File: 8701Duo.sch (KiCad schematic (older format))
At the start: 12 parts, among them J1 Clock, U1 ICS525-01R, U2 MOS8701, U3 74LVC1G06, X1 LFSPXO021772Bulk, X2 LFSPXO020648Bulk

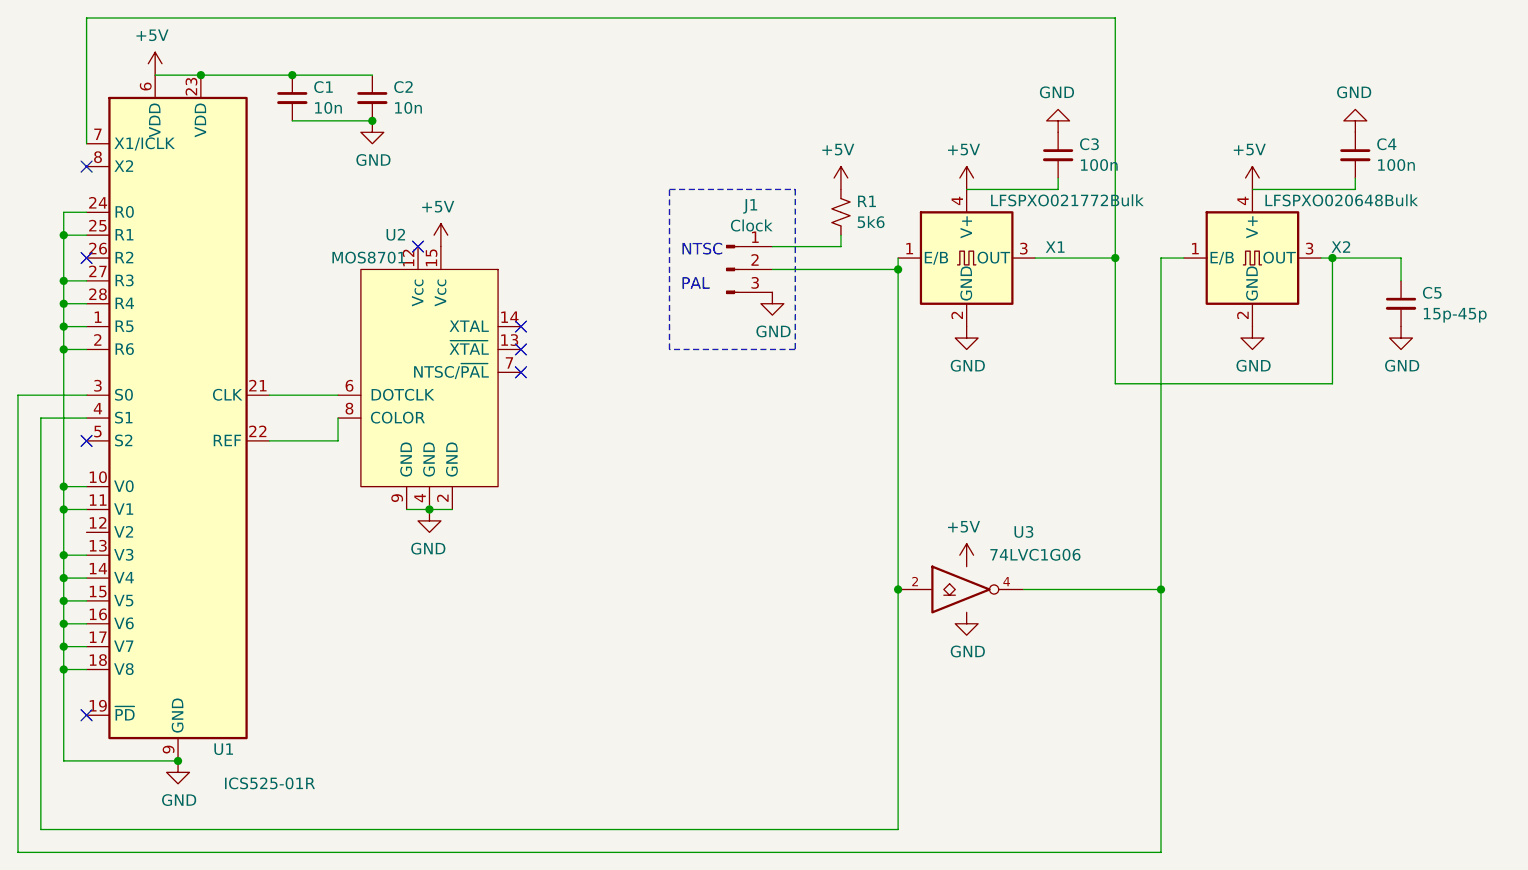
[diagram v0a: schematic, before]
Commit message: Add files via upload
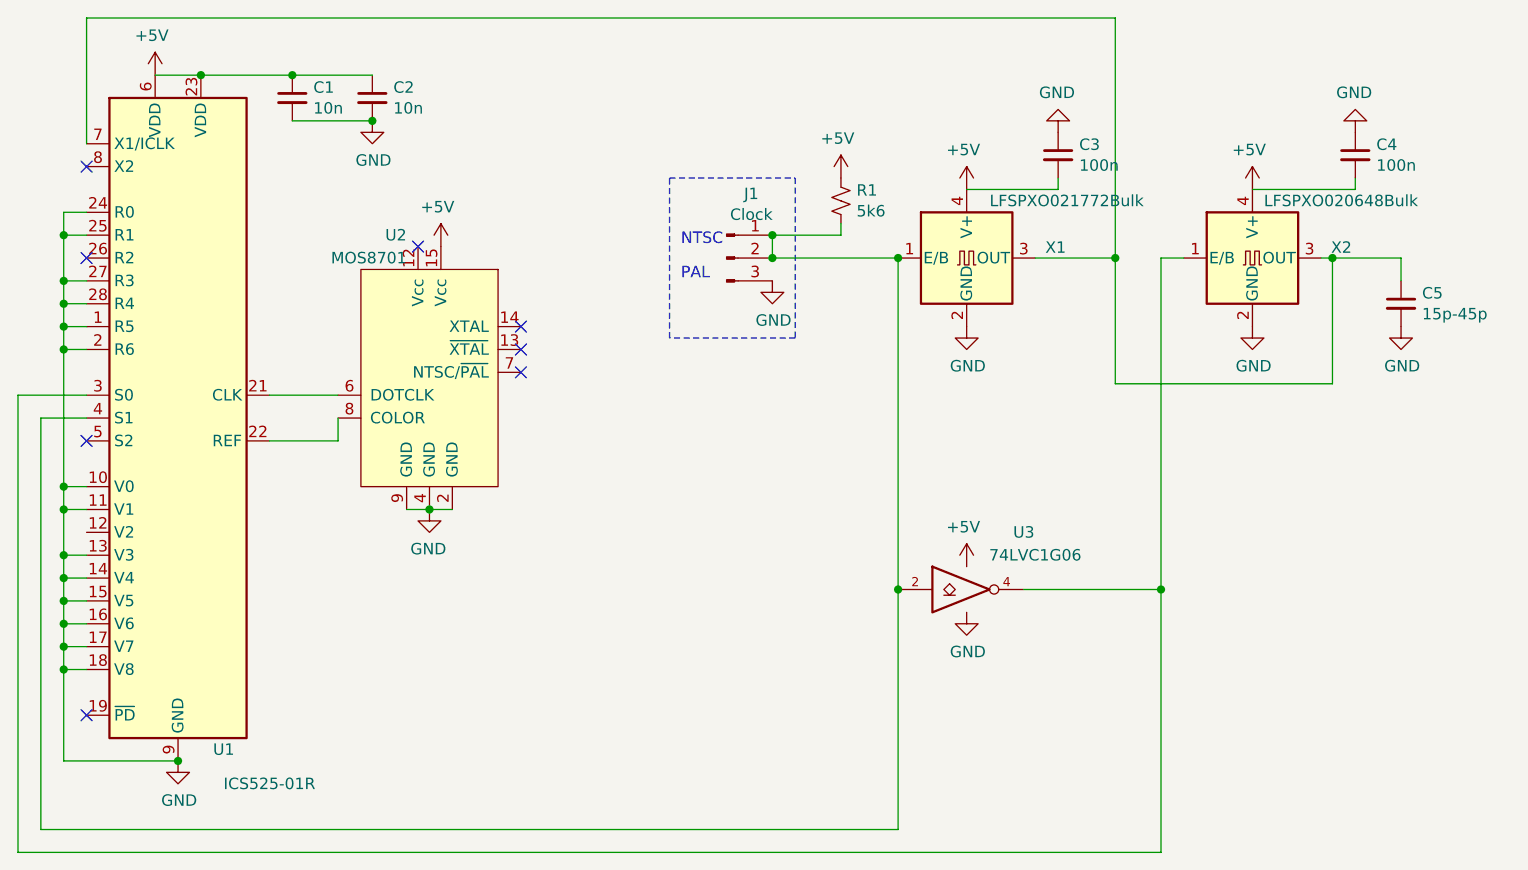
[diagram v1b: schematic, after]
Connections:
- net at J1.2 (Pin_2), U1.4 (S1), U3.2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: now also J1.1 (Pin_1), R1.2
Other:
- moved on the sheet: J1, R1
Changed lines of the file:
@@
 $EndComp
-Wire Wire Line
-	7650 2050 7650 2100
 Wire Wire Line
 	8800 2050 8900 2050
@@
 L Connector:Conn_01x03_Male J1
 U 1 1 5EF16EAC
-P 6900 2100
-F 0 "J1" H 7008 2381 50  0000 C CNN
-F 1 "Clock" H 7008 2290 50  0000 C CNN
-F 2 "Connector_PinHeader_2.54mm:PinHeader_1x03_P2.54mm_Vertical" H 6900 2100 50  0001 C CNN
-F 3 "~" H 6900 2100 50  0001 C CNN
-	1    6900 2100
+P 6900 2050
+F 0 "J1" H 7008 2331 50  0000 C CNN
+F 1 "Clock" H 7008 2240 50  0000 C CNN
+F 2 "Connector_PinHeader_2.54mm:PinHeader_1x03_P2.54mm_Vertical" H 6900 2050 50  0001 C CNN
+F 3 "~" H 6900 2050 50  0001 C CNN
+	1    6900 2050
 	1    0    0    -1
 $EndComp
@@
 L Device:R_Small_US R1
 U 1 1 5EF17D87
-P 7400 1850
-F 0 "R1" H 7468 1896 50  0000 L CNN
-F 1 "5k6" H 7468 1805 50  0000 L CNN
-F 2 "Resistor_SMD:R_0805_2012Metric_Pad1.15x1.40mm_HandSolder" H 7400 1850 50  0001 C CNN
-F 3 "~" H 7400 1850 50  0001 C CNN
-	1    7400 1850
-	1    0    0    -1
-$EndComp
-Wire Wire Line
-	7100 2000 7400 2000
-Wire Wire Line
-	7400 2000 7400 1950
+P 7400 1800
+F 0 "R1" H 7468 1846 50  0000 L CNN
+F 1 "5k6" H 7468 1755 50  0000 L CNN
+F 2 "Resistor_SMD:R_0805_2012Metric_Pad1.15x1.40mm_HandSolder" H 7400 1800 50  0001 C CNN
+F 3 "~" H 7400 1800 50  0001 C CNN
+	1    7400 1800
+	1    0    0    -1
+$EndComp
+Wire Wire Line
+	7100 1950 7400 1950
+Wire Wire Line
+	7400 1950 7400 1900
 $Comp
 L Power2:GND #PWR06
 U 1 1 5EF27873
-P 7100 2200
-F 0 "#PWR06" H 7100 1950 50  0001 C CNN
-F 1 "GND" H 7105 2027 50  0000 C CNN
-F 2 "" H 7100 2200 50  0001 C CNN
-F 3 "" H 7100 2200 50  0001 C CNN
-	1    7100 2200
-	1    0    0    -1
-$EndComp
-Wire Wire Line
-	7100 2100 7650 2100
-Connection ~ 7650 2100
+P 7100 2150
+F 0 "#PWR06" H 7100 1900 50  0001 C CNN
+F 1 "GND" H 7105 1977 50  0000 C CNN
+F 2 "" H 7100 2150 50  0001 C CNN
+F 3 "" H 7100 2150 50  0001 C CNN
+	1    7100 2150
+	1    0    0    -1
+$EndComp
+Wire Wire Line
+	7100 2050 7650 2050
 NoConn ~ 4100 1650
 Wire Wire Line
@@
 	-1   0    0    1
 $EndComp
-Text Notes 6700 2050 0    50   ~ 0
+Text Notes 6700 2000 0    50   ~ 0
 NTSC
-Text Notes 6700 2200 0    50   ~ 0
+Text Notes 6700 2150 0    50   ~ 0
 PAL
 Wire Notes Line
-	6650 1750 7200 1750
+	6650 1700 7200 1700
 Wire Notes Line
-	7200 1750 7200 2450
+	7200 1700 7200 2400
 Wire Notes Line
-	7200 2450 6650 2450
+	7200 2400 6650 2400
 Wire Notes Line
-	6650 2450 6650 1750
+	6650 2400 6650 1700
 $Comp
 L Device:C_Small C1
@@
 	8800 2050 8800 3500
 Wire Wire Line
-	7650 2100 7650 3500
-Wire Wire Line
 	7650 3500 7650 4550
 Wire Wire Line
@@
 L Power2:+5V #PWR07
 U 1 1 5EF07D9E
-P 7400 1750
-F 0 "#PWR07" H 7400 1600 50  0001 C CNN
-F 1 "+5V" H 7415 1923 50  0000 C CNN
-F 2 "" H 7400 1750 50  0001 C CNN
-F 3 "" H 7400 1750 50  0001 C CNN
-	1    7400 1750
+P 7400 1700
+F 0 "#PWR07" H 7400 1550 50  0001 C CNN
+F 1 "+5V" H 7415 1873 50  0000 C CNN
+F 2 "" H 7400 1700 50  0001 C CNN
+F 3 "" H 7400 1700 50  0001 C CNN
+	1    7400 1700
 	-1   0    0    -1
 $EndComp
@@
 	-1   0    0    -1
 $EndComp
+Connection ~ 7650 2050
+Wire Wire Line
+	7650 2050 7650 3500
+Wire Wire Line
+	7100 1950 7100 2050
+Connection ~ 7100 1950
+Connection ~ 7100 2050
 $EndSCHEMATC
